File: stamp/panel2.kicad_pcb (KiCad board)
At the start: 4 copper layers, 80.1 x 80.1 mm, 784 parts, among them IC1 TP4056, Q1 SI2301CDS-T1-GE3, U1 AP2112K-3.3, U2 AP9101CK6, U3 FS8205

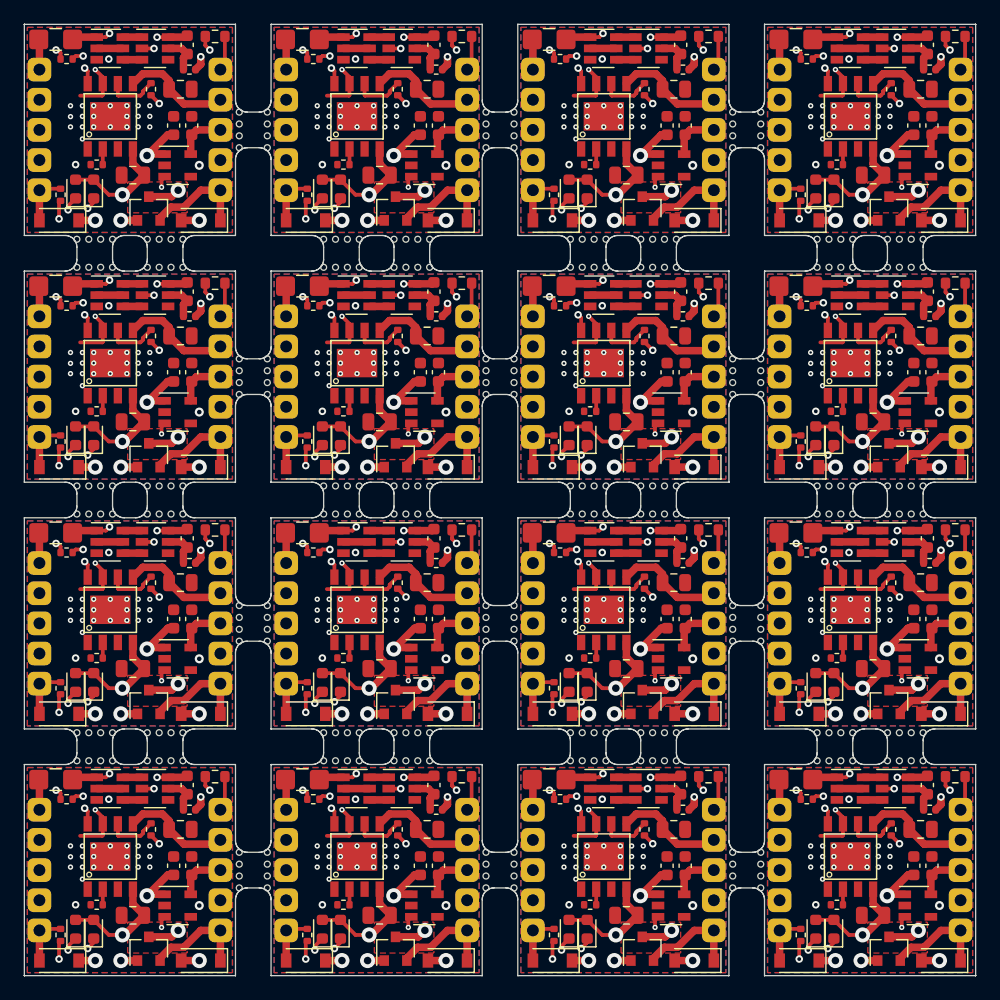
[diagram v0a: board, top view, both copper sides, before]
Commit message: Ordered on 2020-11-30. v0.3.0 release.
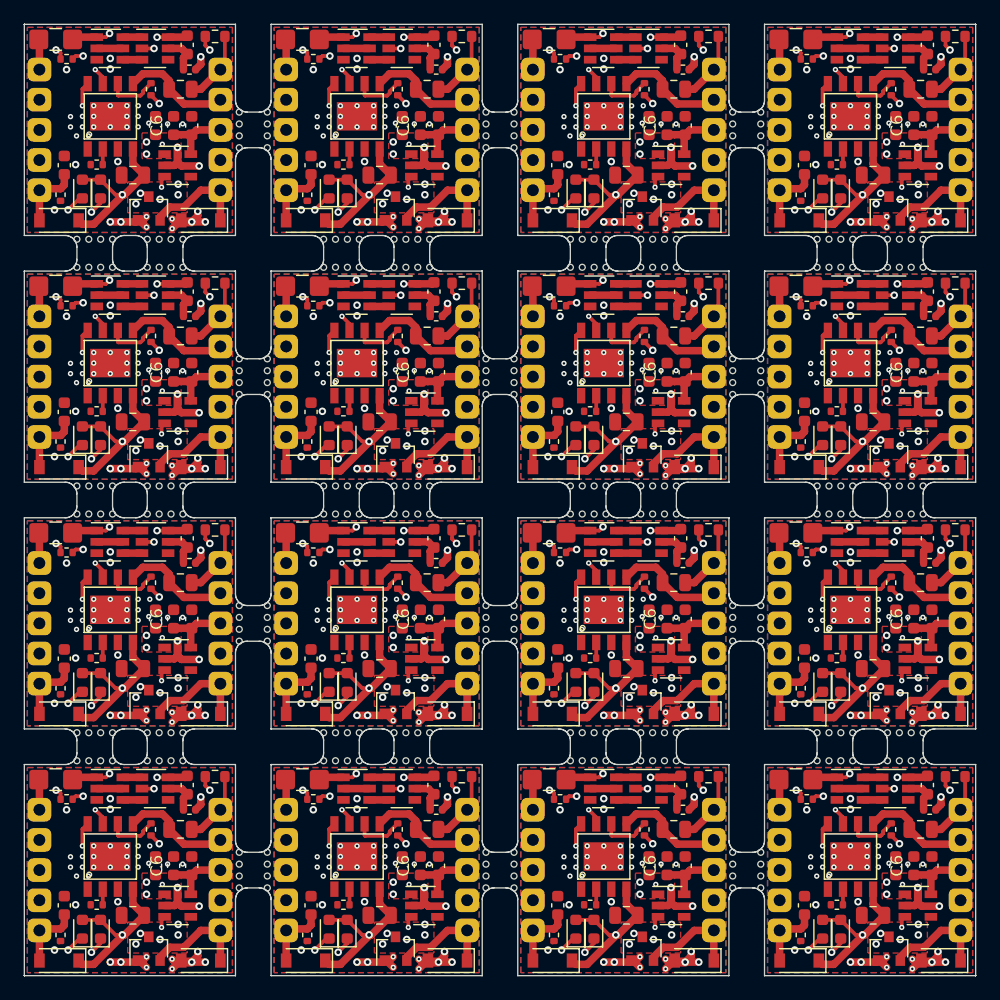
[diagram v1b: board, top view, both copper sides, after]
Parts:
- removed the C3 at (124.9, 120.9)
- removed the C3 at (104.1, 79.3)
- removed the C3 at (83.4, 79.3)
- removed the C3 at (62.6, 79.3)
- removed the C3 at (124.9, 58.5)
- removed the C3 at (104.1, 58.5)
- removed the C3 at (83.4, 58.5)
- removed the C3 at (62.6, 58.5)
- removed the C3 at (104.1, 120.9)
- removed the C3 at (83.4, 120.9)
- removed the C3 at (62.6, 120.9)
- removed the C3 at (124.9, 100.1)
- removed the C3 at (104.1, 100.1)
- removed the C3 at (83.4, 100.1)
- removed the C3 at (62.6, 100.1)
- removed the C3 at (124.9, 79.3)
- removed the D1 at (118.2, 126.2)
- removed the D1 at (97.4, 84.6)
- removed the D1 at (76.6, 84.6)
- removed the D1 at (55.8, 84.6)
- removed the D1 at (118.2, 63.9)
- removed the D1 at (97.4, 63.9)
- removed the D1 at (76.6, 63.9)
- removed the D1 at (55.8, 63.9)
- removed the D1 at (97.4, 126.2)
- removed the D1 at (76.6, 126.2)
- removed the D1 at (55.8, 126.2)
- removed the D1 at (118.2, 105.4)
- removed the D1 at (97.4, 105.4)
- removed the D1 at (76.6, 105.4)
- removed the D1 at (55.8, 105.4)
- removed the D1 at (118.2, 84.6)
- removed the D2 at (116.7, 126.2)
- removed the D2 at (95.9, 84.6)
- removed the D2 at (75.1, 84.6)
- removed the D2 at (54.3, 84.6)
- removed the D2 at (116.7, 63.9)
- removed the D2 at (95.9, 63.9)
- removed the D2 at (75.1, 63.9)
- removed the D2 at (54.3, 63.9)
- removed the D2 at (95.9, 126.2)
- removed the D2 at (75.1, 126.2)
- removed the D2 at (54.3, 126.2)
- removed the D2 at (116.7, 105.4)
- removed the D2 at (95.9, 105.4)
- removed the D2 at (75.1, 105.4)
- removed the D2 at (54.3, 105.4)
- removed the D2 at (116.7, 84.6)
- added C3: 1uF, Capacitor_SMD:C_0603_1608Metric, F.Cu at (123.4, 120.9)
- added C3: 1uF, Capacitor_SMD:C_0603_1608Metric, F.Cu at (102.6, 79.3)
- added C3: 1uF, Capacitor_SMD:C_0603_1608Metric, F.Cu at (81.8, 79.3)
- added C3: 1uF, Capacitor_SMD:C_0603_1608Metric, F.Cu at (61.0, 79.3)
- added C3: 1uF, Capacitor_SMD:C_0603_1608Metric, F.Cu at (123.4, 58.5)
- added C3: 1uF, Capacitor_SMD:C_0603_1608Metric, F.Cu at (102.6, 58.5)
- added C3: 1uF, Capacitor_SMD:C_0603_1608Metric, F.Cu at (81.8, 58.5)
- added C3: 1uF, Capacitor_SMD:C_0603_1608Metric, F.Cu at (61.0, 58.5)
- added C3: 1uF, Capacitor_SMD:C_0603_1608Metric, F.Cu at (102.6, 120.9)
- added C3: 1uF, Capacitor_SMD:C_0603_1608Metric, F.Cu at (81.8, 120.9)
- added C3: 1uF, Capacitor_SMD:C_0603_1608Metric, F.Cu at (61.0, 120.9)
- added C3: 1uF, Capacitor_SMD:C_0603_1608Metric, F.Cu at (123.4, 100.1)
- added C3: 1uF, Capacitor_SMD:C_0603_1608Metric, F.Cu at (102.6, 100.1)
- added C3: 1uF, Capacitor_SMD:C_0603_1608Metric, F.Cu at (81.8, 100.1)
- added C3: 1uF, Capacitor_SMD:C_0603_1608Metric, F.Cu at (61.0, 100.1)
- added C3: 1uF, Capacitor_SMD:C_0603_1608Metric, F.Cu at (123.4, 79.3)
- added C6: 1uF, Capacitor_SMD:C_0603_1608Metric, F.Cu at (124.9, 120.9)
- added C6: 1uF, Capacitor_SMD:C_0603_1608Metric, F.Cu at (104.1, 79.3)
- added C6: 1uF, Capacitor_SMD:C_0603_1608Metric, F.Cu at (83.4, 79.3)
- added C6: 1uF, Capacitor_SMD:C_0603_1608Metric, F.Cu at (62.6, 79.3)
- added C6: 1uF, Capacitor_SMD:C_0603_1608Metric, F.Cu at (124.9, 58.5)
- added C6: 1uF, Capacitor_SMD:C_0603_1608Metric, F.Cu at (104.1, 58.5)
- added C6: 1uF, Capacitor_SMD:C_0603_1608Metric, F.Cu at (83.4, 58.5)
- added C6: 1uF, Capacitor_SMD:C_0603_1608Metric, F.Cu at (62.6, 58.5)
- added C6: 1uF, Capacitor_SMD:C_0603_1608Metric, F.Cu at (104.1, 120.9)
- added C6: 1uF, Capacitor_SMD:C_0603_1608Metric, F.Cu at (83.4, 120.9)
- added C6: 1uF, Capacitor_SMD:C_0603_1608Metric, F.Cu at (62.6, 120.9)
- added C6: 1uF, Capacitor_SMD:C_0603_1608Metric, F.Cu at (124.9, 100.1)
- added C6: 1uF, Capacitor_SMD:C_0603_1608Metric, F.Cu at (104.1, 100.1)
- added C6: 1uF, Capacitor_SMD:C_0603_1608Metric, F.Cu at (83.4, 100.1)
- added C6: 1uF, Capacitor_SMD:C_0603_1608Metric, F.Cu at (62.6, 100.1)
- added C6: 1uF, Capacitor_SMD:C_0603_1608Metric, F.Cu at (124.9, 79.3)
- added C7: 1uF, Capacitor_SMD:C_0603_1608Metric, F.Cu at (115.7, 124.2)
- added C7: 1uF, Capacitor_SMD:C_0603_1608Metric, F.Cu at (94.9, 82.6)
- added C7: 1uF, Capacitor_SMD:C_0603_1608Metric, F.Cu at (74.1, 82.6)
- added C7: 1uF, Capacitor_SMD:C_0603_1608Metric, F.Cu at (53.4, 82.6)
- added C7: 1uF, Capacitor_SMD:C_0603_1608Metric, F.Cu at (115.7, 61.9)
- added C7: 1uF, Capacitor_SMD:C_0603_1608Metric, F.Cu at (94.9, 61.9)
- added C7: 1uF, Capacitor_SMD:C_0603_1608Metric, F.Cu at (74.1, 61.9)
- added C7: 1uF, Capacitor_SMD:C_0603_1608Metric, F.Cu at (53.4, 61.9)
- added C7: 1uF, Capacitor_SMD:C_0603_1608Metric, F.Cu at (94.9, 124.2)
- added C7: 1uF, Capacitor_SMD:C_0603_1608Metric, F.Cu at (74.1, 124.2)
- added C7: 1uF, Capacitor_SMD:C_0603_1608Metric, F.Cu at (53.4, 124.2)
- added C7: 1uF, Capacitor_SMD:C_0603_1608Metric, F.Cu at (115.7, 103.4)
- added C7: 1uF, Capacitor_SMD:C_0603_1608Metric, F.Cu at (94.9, 103.4)
- added C7: 1uF, Capacitor_SMD:C_0603_1608Metric, F.Cu at (74.1, 103.4)
- added C7: 1uF, Capacitor_SMD:C_0603_1608Metric, F.Cu at (53.4, 103.4)
- added C7: 1uF, Capacitor_SMD:C_0603_1608Metric, F.Cu at (115.7, 82.6)
- added D1: GREEN, LED_SMD:LED_0603_1608Metric, F.Cu at (118.8, 126.2)
- added D1: GREEN, LED_SMD:LED_0603_1608Metric, F.Cu at (98.0, 84.6)
- added D1: GREEN, LED_SMD:LED_0603_1608Metric, F.Cu at (77.2, 84.6)
- added D1: GREEN, LED_SMD:LED_0603_1608Metric, F.Cu at (56.4, 84.6)
- added D1: GREEN, LED_SMD:LED_0603_1608Metric, F.Cu at (118.8, 63.9)
- added D1: GREEN, LED_SMD:LED_0603_1608Metric, F.Cu at (98.0, 63.9)
- added D1: GREEN, LED_SMD:LED_0603_1608Metric, F.Cu at (77.2, 63.9)
- added D1: GREEN, LED_SMD:LED_0603_1608Metric, F.Cu at (56.4, 63.9)
- added D1: GREEN, LED_SMD:LED_0603_1608Metric, F.Cu at (98.0, 126.2)
- added D1: GREEN, LED_SMD:LED_0603_1608Metric, F.Cu at (77.2, 126.2)
- added D1: GREEN, LED_SMD:LED_0603_1608Metric, F.Cu at (56.4, 126.2)
- added D1: GREEN, LED_SMD:LED_0603_1608Metric, F.Cu at (118.8, 105.4)
- added D1: GREEN, LED_SMD:LED_0603_1608Metric, F.Cu at (98.0, 105.4)
- added D1: GREEN, LED_SMD:LED_0603_1608Metric, F.Cu at (77.2, 105.4)
- added D1: GREEN, LED_SMD:LED_0603_1608Metric, F.Cu at (56.4, 105.4)
- added D1: GREEN, LED_SMD:LED_0603_1608Metric, F.Cu at (118.8, 84.6)
- added D2: RED, LED_SMD:LED_0603_1608Metric, F.Cu at (117.2, 126.2)
- added D2: RED, LED_SMD:LED_0603_1608Metric, F.Cu at (96.4, 84.6)
- added D2: RED, LED_SMD:LED_0603_1608Metric, F.Cu at (75.7, 84.6)
- added D2: RED, LED_SMD:LED_0603_1608Metric, F.Cu at (54.9, 84.6)
- added D2: RED, LED_SMD:LED_0603_1608Metric, F.Cu at (117.2, 63.9)
- added D2: RED, LED_SMD:LED_0603_1608Metric, F.Cu at (96.4, 63.9)
- added D2: RED, LED_SMD:LED_0603_1608Metric, F.Cu at (75.7, 63.9)
- added D2: RED, LED_SMD:LED_0603_1608Metric, F.Cu at (54.9, 63.9)
- added D2: RED, LED_SMD:LED_0603_1608Metric, F.Cu at (96.4, 126.2)
- added D2: RED, LED_SMD:LED_0603_1608Metric, F.Cu at (75.7, 126.2)
- added D2: RED, LED_SMD:LED_0603_1608Metric, F.Cu at (54.9, 126.2)
- added D2: RED, LED_SMD:LED_0603_1608Metric, F.Cu at (117.2, 105.4)
- added D2: RED, LED_SMD:LED_0603_1608Metric, F.Cu at (96.4, 105.4)
- added D2: RED, LED_SMD:LED_0603_1608Metric, F.Cu at (75.7, 105.4)
- added D2: RED, LED_SMD:LED_0603_1608Metric, F.Cu at (54.9, 105.4)
- added D2: RED, LED_SMD:LED_0603_1608Metric, F.Cu at (117.2, 84.6)
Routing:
- net Board_16-/+BATT: track 43.0 -> 20.3 mm, vias 2 -> 6
- net Board_4-/+BATT: track 43.0 -> 20.3 mm, vias 2 -> 6
- net Board_13-/+BATT: track 43.0 -> 20.3 mm, vias 2 -> 6
- net Board_14-/+BATT: track 43.0 -> 20.3 mm, vias 2 -> 6
- net Board_1-/+BATT: track 43.0 -> 20.3 mm, vias 2 -> 6
- net Board_2-/+BATT: track 43.0 -> 20.3 mm, vias 2 -> 6
- net Board_15-/+BATT: track 43.0 -> 20.3 mm, vias 2 -> 6
- net Board_8-/+BATT: track 43.0 -> 20.3 mm, vias 2 -> 6
- net Board_3-/+BATT: track 43.0 -> 20.3 mm, vias 2 -> 6
- net Board_12-/+BATT: track 43.0 -> 20.3 mm, vias 2 -> 6
- net Board_9-/+BATT: track 43.0 -> 20.3 mm, vias 2 -> 6
- net Board_6-/+BATT: track 43.0 -> 20.3 mm, vias 2 -> 6
- net Board_5-/+BATT: track 43.0 -> 20.3 mm, vias 2 -> 6
- net Board_10-/+BATT: track 43.0 -> 20.3 mm, vias 2 -> 6
- net Board_7-/+BATT: track 43.0 -> 20.3 mm, vias 2 -> 6
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- added copper zone on In2.Cu, net Board_1-/+BATT
- added copper zone on In2.Cu, net Board_1-/+CHARGE
- added copper zone on F.Cu, net Board_1-/VMAX
- added copper zone on In1.Cu, net Board_1-/VMAX
- added copper zone on In2.Cu, net Board_10-/+BATT
- added copper zone on In2.Cu, net Board_10-/+CHARGE
- added copper zone on F.Cu, net Board_10-/VMAX
- added copper zone on In1.Cu, net Board_10-/VMAX
- added copper zone on In2.Cu, net Board_11-/+BATT
- added copper zone on In2.Cu, net Board_11-/+CHARGE
- added copper zone on F.Cu, net Board_11-/VMAX
- added copper zone on In1.Cu, net Board_11-/VMAX
- added copper zone on In2.Cu, net Board_12-/+BATT
- added copper zone on In2.Cu, net Board_12-/+CHARGE
- added copper zone on F.Cu, net Board_12-/VMAX
- added copper zone on In1.Cu, net Board_12-/VMAX
- added copper zone on In2.Cu, net Board_13-/+BATT
- added copper zone on In2.Cu, net Board_13-/+CHARGE
- added copper zone on F.Cu, net Board_13-/VMAX
- added copper zone on In1.Cu, net Board_13-/VMAX
- added copper zone on In2.Cu, net Board_14-/+BATT
- added copper zone on In2.Cu, net Board_14-/+CHARGE
- added copper zone on F.Cu, net Board_14-/VMAX
- added copper zone on In1.Cu, net Board_14-/VMAX
- added copper zone on In2.Cu, net Board_15-/+BATT
- added copper zone on In2.Cu, net Board_15-/+CHARGE
- added copper zone on F.Cu, net Board_15-/VMAX
- added copper zone on In1.Cu, net Board_15-/VMAX
- added copper zone on In2.Cu, net Board_16-/+BATT
- added copper zone on In2.Cu, net Board_16-/+CHARGE
- added copper zone on F.Cu, net Board_16-/VMAX
- added copper zone on In1.Cu, net Board_16-/VMAX
- added copper zone on In2.Cu, net Board_2-/+BATT
- added copper zone on In2.Cu, net Board_2-/+CHARGE
- added copper zone on F.Cu, net Board_2-/VMAX
- added copper zone on In1.Cu, net Board_2-/VMAX
- added copper zone on In2.Cu, net Board_3-/+BATT
- added copper zone on In2.Cu, net Board_3-/+CHARGE
- added copper zone on F.Cu, net Board_3-/VMAX
- added copper zone on In1.Cu, net Board_3-/VMAX
- added copper zone on In2.Cu, net Board_4-/+BATT
- added copper zone on In2.Cu, net Board_4-/+CHARGE
- added copper zone on F.Cu, net Board_4-/VMAX
- added copper zone on In1.Cu, net Board_4-/VMAX
- added copper zone on In2.Cu, net Board_5-/+BATT
- added copper zone on In2.Cu, net Board_5-/+CHARGE
- added copper zone on F.Cu, net Board_5-/VMAX
- added copper zone on In1.Cu, net Board_5-/VMAX
- added copper zone on In2.Cu, net Board_6-/+BATT
- added copper zone on In2.Cu, net Board_6-/+CHARGE
- added copper zone on F.Cu, net Board_6-/VMAX
- added copper zone on In1.Cu, net Board_6-/VMAX
- added copper zone on In2.Cu, net Board_7-/+BATT
- added copper zone on In2.Cu, net Board_7-/+CHARGE
- added copper zone on F.Cu, net Board_7-/VMAX
- added copper zone on In1.Cu, net Board_7-/VMAX
- added copper zone on In2.Cu, net Board_8-/+BATT
- added copper zone on In2.Cu, net Board_8-/+CHARGE
- added copper zone on F.Cu, net Board_8-/VMAX
- added copper zone on In1.Cu, net Board_8-/VMAX
- added copper zone on In2.Cu, net Board_9-/+BATT
- added copper zone on In2.Cu, net Board_9-/+CHARGE
- added copper zone on F.Cu, net Board_9-/VMAX
- added copper zone on In1.Cu, net Board_9-/VMAX
